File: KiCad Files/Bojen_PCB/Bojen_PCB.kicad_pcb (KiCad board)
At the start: 2 copper layers, 201.9 x 114.3 mm, 9 parts, among them J1 5V Power In, J2 Battery Voltage, U1 Display_TFT_1.8Zoll_ST7735, U2 NEO-GPS8M, U3 SIM800L-CORE, U4 TLP5110 Adafruit Modul, U5 ADS1115 Module, U6 PCF8575 Module, U7 ESP32-DEVKIT-V1

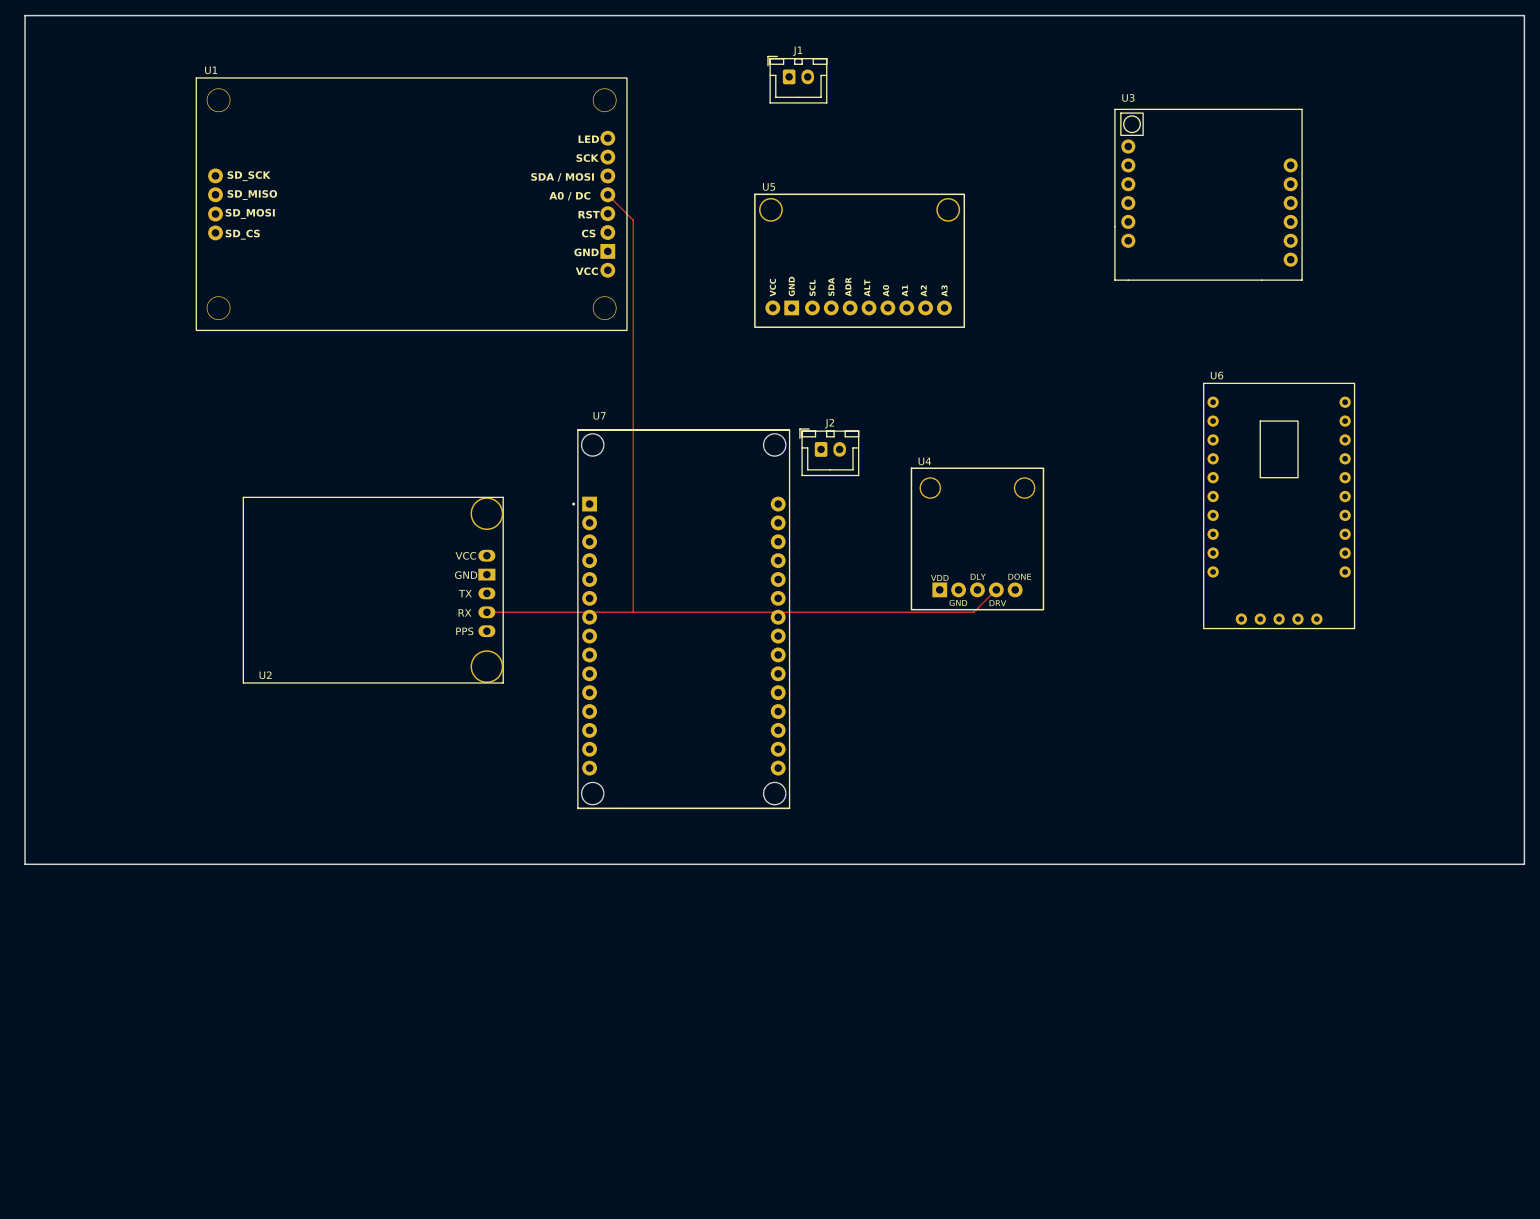
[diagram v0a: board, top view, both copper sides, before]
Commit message: layout
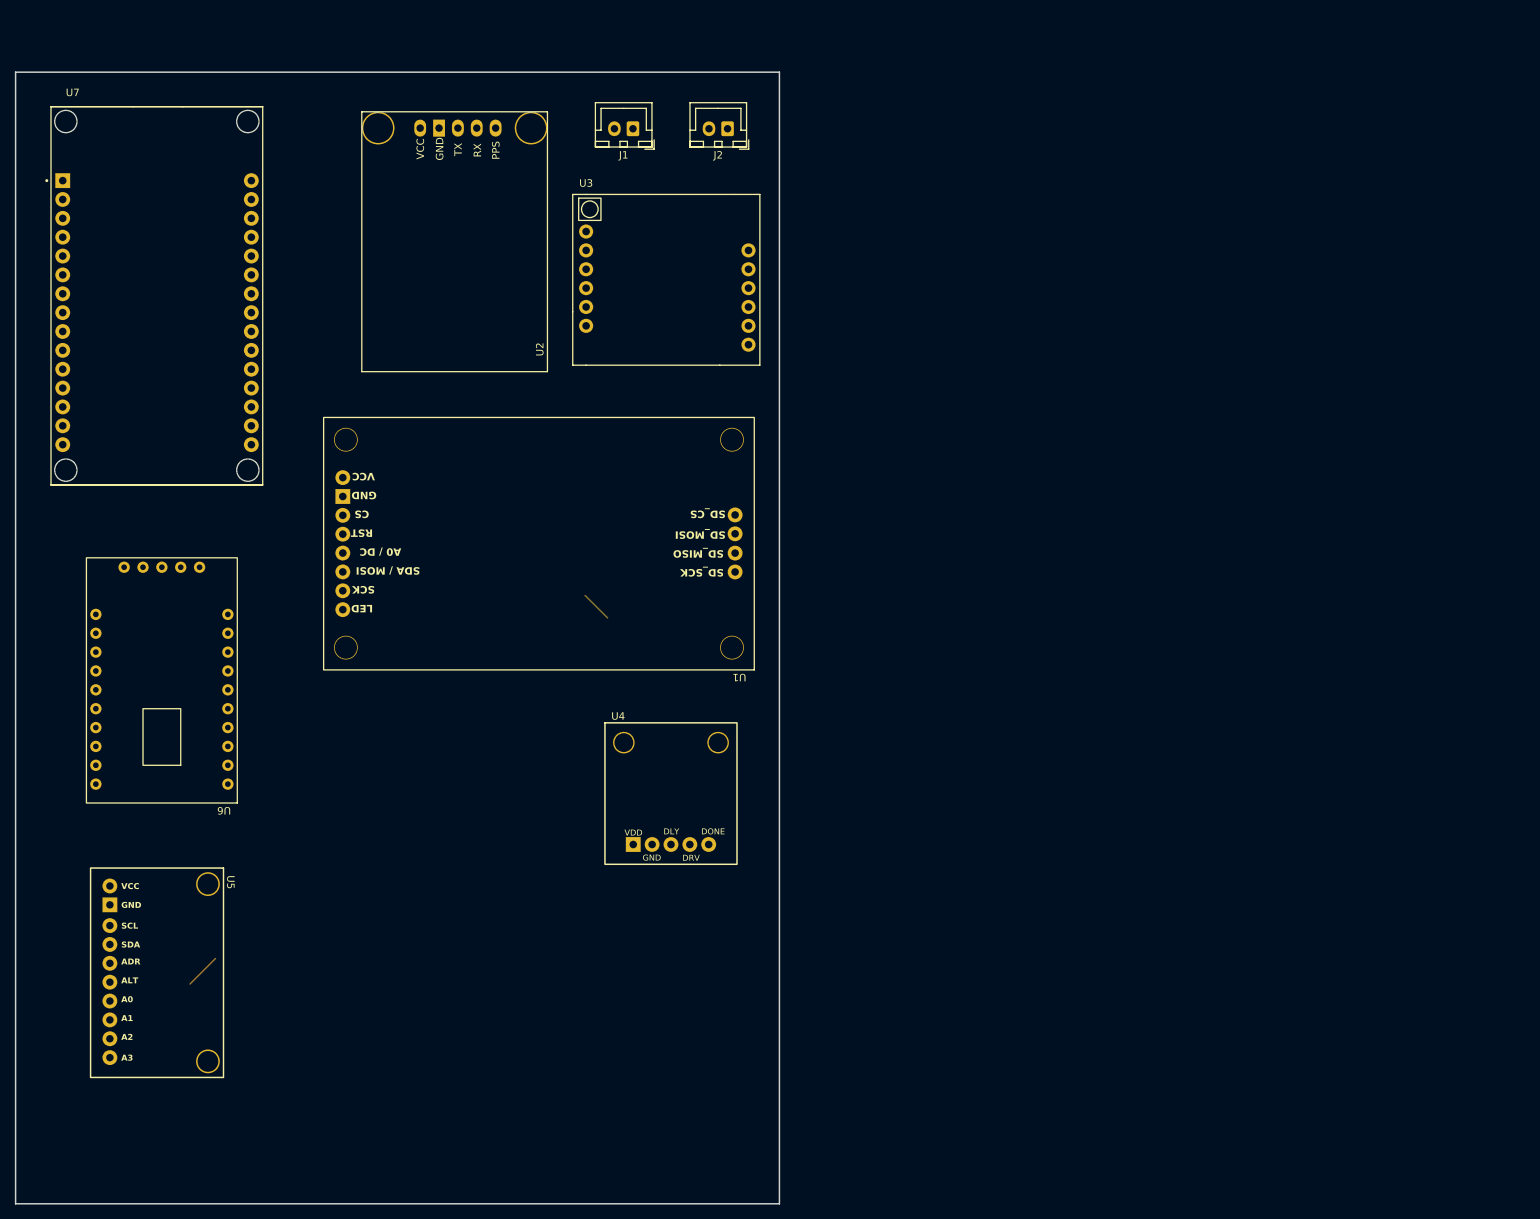
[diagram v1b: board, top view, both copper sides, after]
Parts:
- moved U6 139.6 mm to (69.2, 122.6), turned to 180 degrees
- moved U5 134.7 mm to (57.1, 145.4), turned to -90 degrees
- moved U7 83.3 mm to (57.1, 54.2)
- moved U2 77.2 mm to (109.7, 29.5), turned to 90 degrees
- moved U3 73.9 mm to (114.9, 45.6)
- moved U4 53.7 mm to (126.4, 121.3)
- moved U1 48.8 mm to (108.6, 87.6), turned to 180 degrees
- moved J2 45.0 mm to (134.0, 31.8), turned to 180 degrees
- moved J1 22.2 mm to (121.2, 31.8), turned to 180 degrees
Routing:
- net (no net): track 127.5 -> 0.00 mm
- net unconnected-(U1-TFT_A0_DC-Pad4): track 0.00 -> 4.85 mm
- net Net-(U4-DRV): track 0.00 -> 4.27 mm
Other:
- board size 201.9 x 114.3 mm -> 102.9 x 152.4 mm

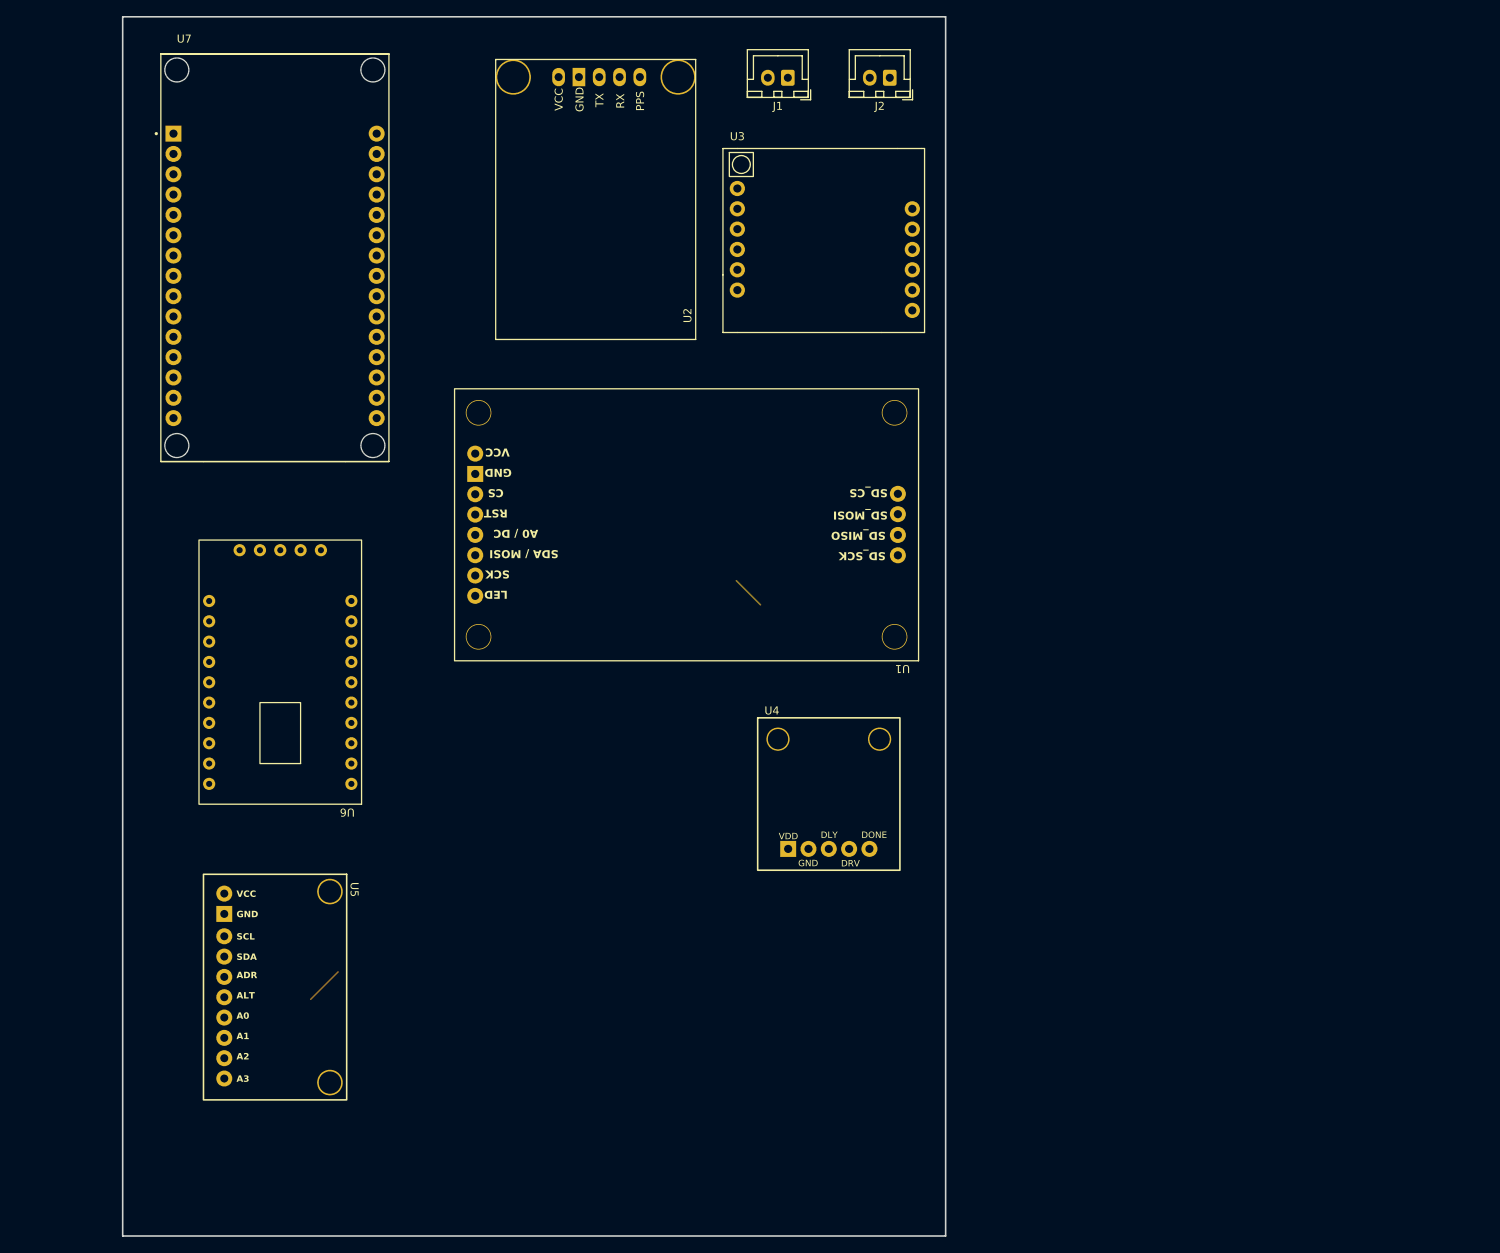
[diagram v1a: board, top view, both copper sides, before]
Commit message: PCB Design
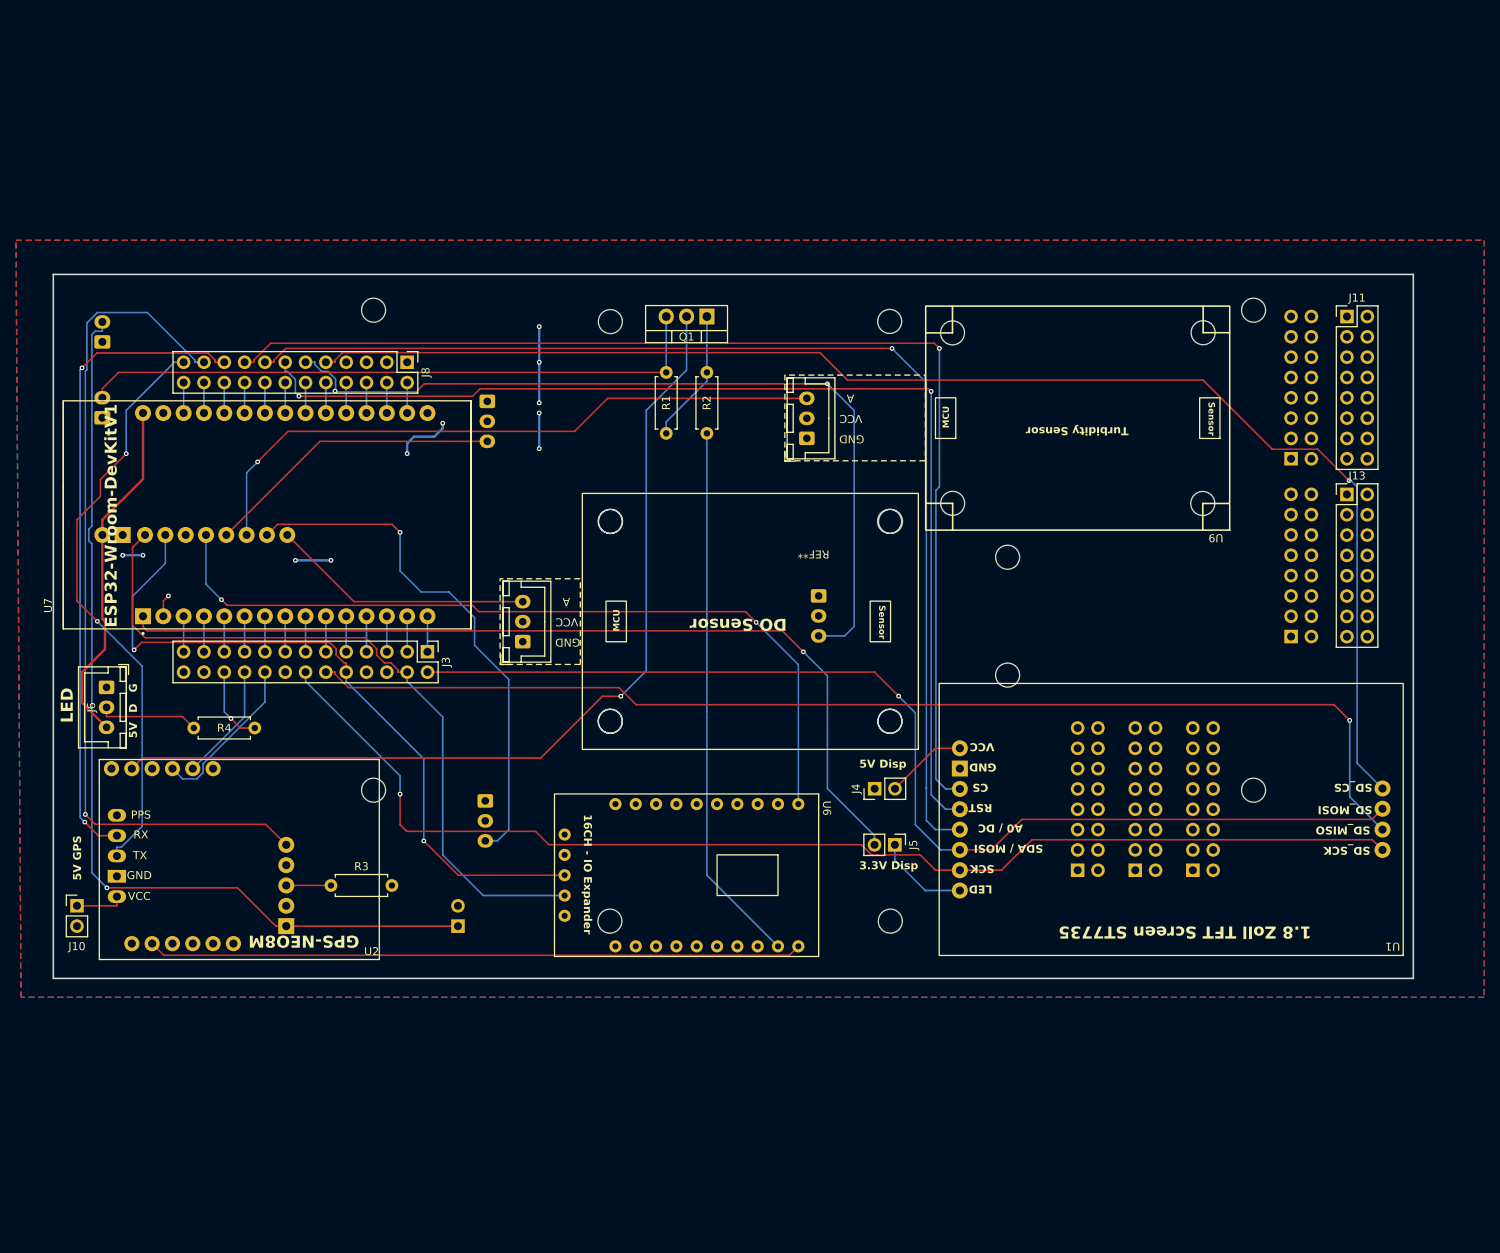
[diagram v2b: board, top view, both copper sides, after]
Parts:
- added J10: GPS EN, Connector_PinHeader_2.54mm:PinHeader_1x02_P2.54mm_Vertical, F.Cu at (32.4, 135.3)
- added J11: Conn_02x08_Odd_Even, Connector_PinHeader_2.54mm:PinHeader_2x08_P2.54mm_Vertical, F.Cu at (191.1, 61.6)
- added J13: Conn_02x08_Odd_Even, Connector_PinHeader_2.54mm:PinHeader_2x08_P2.54mm_Vertical, F.Cu at (191.1, 83.8)
- added J14: Conn_02x08_Odd_Even, Connector_PinHeader_2.54mm:PinHeader_2x08_P2.54mm_Vertical, B.Cu at (184.2, 101.6)
- added J15: Conn_02x08_Odd_Even, Connector_PinHeader_2.54mm:PinHeader_2x08_P2.54mm_Vertical, B.Cu at (184.2, 79.4)
- added J16: Conn_02x08_Odd_Even, Connector_PinHeader_2.54mm:PinHeader_2x08_P2.54mm_Vertical, B.Cu at (157.5, 130.8)
- added J17: Conn_02x08_Odd_Even, Connector_PinHeader_2.54mm:PinHeader_2x08_P2.54mm_Vertical, B.Cu at (164.7, 130.8)
- added J18: Conn_02x08_Odd_Even, Connector_PinHeader_2.54mm:PinHeader_2x08_P2.54mm_Vertical, B.Cu at (171.9, 130.8)
- added J3: GPIO Breakout 2, Connector_PinHeader_2.54mm:PinHeader_2x13_P2.54mm_Vertical, F.Cu at (76.2, 103.5)
- added J4: 5V TFT, Connector_PinHeader_2.54mm:PinHeader_1x02_P2.54mm_Vertical, F.Cu at (132.1, 120.6)
- added J5: 3.3V TFT, Connector_PinHeader_2.54mm:PinHeader_1x02_P2.54mm_Vertical, F.Cu at (134.6, 127.6)
- added J6: LED, Connector_JST:JST_XH_B3B-XH-A_1x03_P2.50mm_Vertical, F.Cu at (36.1, 108.0)
- added J8: GPIO Breakout 1, Connector_PinHeader_2.54mm:PinHeader_2x12_P2.54mm_Vertical, F.Cu at (73.7, 67.3)
- added J9: PWR TMR SKIP, Connector_PinHeader_2.54mm:PinHeader_1x02_P2.54mm_Vertical, B.Cu at (80.0, 137.8)
- added Q1: IRF5210PBF, Package_TO_SOT_THT:TO-220-3_Vertical, F.Cu at (111.1, 61.6)
- added R1: 10k, Resistor_THT:R_Axial_DIN0207_L6.3mm_D2.5mm_P7.62mm_Horizontal, F.Cu at (106.0, 68.6)
- added R2: 470, Resistor_THT:R_Axial_DIN0207_L6.3mm_D2.5mm_P7.62mm_Horizontal, F.Cu at (111.1, 76.2)
- added R3: 220k, Resistor_THT:R_Axial_DIN0207_L6.3mm_D2.5mm_P7.62mm_Horizontal, F.Cu at (64.1, 132.7)
- added R4: 330, Resistor_THT:R_Axial_DIN0207_L6.3mm_D2.5mm_P7.62mm_Horizontal, F.Cu at (47.0, 113.0)
- added REF**: Battery Footprint, Datenbojen:Battery Footprint, F.Cu at (124.5, 90.8)
- added U10: PH Sensor, Datenbojen:PH Sensor DFRobot, B.Cu at (116.5, 124.7)
- added U11: DO Sensor, Datenbojen:DO Sensor DFRobot, F.Cu at (116.6, 99.7)
- added U12: TMP Sensor, Datenbojen:Tempterature Sensor DFRobot, B.Cu at (153.5, 99.0)
- added U8: TDS Sensor, Datenbojen:TDS Sensor DFRobot, B.Cu at (116.5, 74.7)
- added U9: Turbidity Sensor, Datenbojen:Turbidity Sensor DFRobot, F.Cu at (157.5, 74.3)
- J1, J2, U3: moved to B.Cu
- U1: footprint Datenbojen:ST7735 TFT Screen 1.8 Zoll -> Datenbojen:ST7735 TFT Screen 1.8 Zoll no hole
- U2: footprint Datenbojen:GY-NEO8MV2 -> Datenbojen:GY-NEO8MV2 no hole
- U4: value TLP5110 Adafruit Modul -> TLP5110 Power Timer Modul; footprint Datenbojen:TPL5110 Board -> Datenbojen:TPL5110 Board no hole; moved to B.Cu
- U5: value ADS1115 Module -> ADC - ADS1115 Module; footprint Datenbojen:ADS1115 Module -> Datenbojen:ADC - ADS1115 Module no hole; moved to B.Cu
- U7: footprint Datenbojen:MODULE_ESP32_DEVKIT_V1 -> Datenbojen:MODULE_ESP32_DEVKIT_V1 no hole
- moved U2 115.0 mm to (35.2, 117.0), turned to 180 degrees
- moved J2 107.2 mm to (35.6, 74.3), turned to 90 degrees
- moved U3 106.7 mm to (36.7, 118.1), turned to -90 degrees
- moved J1 91.8 mm to (35.6, 64.8), turned to 90 degrees
- moved U1 70.9 mm to (169.2, 124.5)
- moved U4 62.0 mm to (65.4, 132.7), turned to 90 degrees
- moved U6 55.9 mm to (125.1, 120.0), turned to -90 degrees
- moved U5 51.1 mm to (47.2, 95.2), turned to 0 degrees
- moved U7 32.1 mm to (56.2, 86.4), turned to 90 degrees
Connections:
- J2 pad 1: unconnected-(J2-Pin_1-Pad1) -> GND
- J2 pad 2: unconnected-(J2-Pin_2-Pad2) -> +BATT
- U1 pad 1: unconnected-(U1-TFT_LED-Pad1) -> Net-(J5-Pin_1)
- U1 pad 10: unconnected-(U1-SD_MOSI-Pad10) -> /SPI_MOSI
- U1 pad 11: unconnected-(U1-SD_MISO-Pad11) -> /SPI_MISO
- U1 pad 12: unconnected-(U1-SD_SCK-Pad12) -> /SPI_SCK
- U1 pad 2: unconnected-(U1-TFT_SCK-Pad2) -> /SPI_SCK
- U1 pad 3: unconnected-(U1-TFT_SDA_MOSI-Pad3) -> /SPI_MOSI
- U1 pad 4: unconnected-(U1-TFT_A0_DC-Pad4) -> /TFT_DC
- U1 pad 5: unconnected-(U1-TFT_RST-Pad5) -> /TFT_RST
- U1 pad 6: unconnected-(U1-TFT_CS-Pad6) -> /TFT_CS
- U1 pad 7: unconnected-(U1-GND-Pad7) -> GND
- U1 pad 8: unconnected-(U1-VCC-Pad8) -> Net-(J4-Pin_2)
- U1 pad 9: unconnected-(U1-SD_CS-Pad9) -> /SD_CS
- U2 pad 1: unconnected-(U2-VCC-Pad1) -> Net-(J10-Pin_1)
- U2 pad 2: unconnected-(U2-GND-Pad2) -> GND
- U2 pad 3: unconnected-(U2-TX-Pad3) -> /RX1
- U2 pad 4: unconnected-(U2-RX-Pad4) -> /TX1
- U3 pad 11: unconnected-(U3-DTR-Pad11) -> /SIM_DTR
- U3 pad 2: unconnected-(U3-VCC-Pad2) -> Net-(Q1-D)
- U3 pad 4: unconnected-(U3-RXD-Pad4) -> /TX2
- U3 pad 5: unconnected-(U3-TXD-Pad5) -> /RX2
- U3 pad 6: unconnected-(U3-GND-Pad6) -> GND
- U4 pad 3: unconnected-(U4-Delay-Pad3) -> Net-(U4-Delay)
- U4 pad 4: Net-(U4-DRV) -> +5V
- U4 pad 5: unconnected-(U4-Done-Pad5) -> /PWR_Done
- U5 pad 1: unconnected-(U5-VCC-Pad1) -> +5V
- U5 pad 10: unconnected-(U5-A3-Pad10) -> /ADC3
- U5 pad 2: unconnected-(U5-GND-Pad2) -> GND
- U5 pad 3: unconnected-(U5-SCL-Pad3) -> /I2C_SCL
- U5 pad 4: unconnected-(U5-SDA-Pad4) -> /I2C_SDA
- U5 pad 6: unconnected-(U5-ALRT-Pad6) -> /ADC_ALRT
- U5 pad 7: unconnected-(U5-A0-Pad7) -> /ADC0
- U5 pad 8: unconnected-(U5-A1-Pad8) -> /ADC1
- U5 pad 9: unconnected-(U5-A2-Pad9) -> /ADC2
- U6 pad 1: unconnected-(U6-P10-Pad1) -> /ADC_ALRT
- U6 pad 19: unconnected-(U6-P06-Pad19) -> /~SIM_EN
- U6 pad 20: unconnected-(U6-P07-Pad20) -> /SIM_DTR
- U6 pad C1: unconnected-(U6-GND-PadC1) -> GND
- U6 pad C2: unconnected-(U6-VCC-PadC2) -> +5V
- U6 pad C3: unconnected-(U6-SDA-PadC3) -> /I2C_SDA
- U6 pad C4: unconnected-(U6-SCL-PadC4) -> /I2C_SCL
- U7 pad 1: unconnected-(U7-3V3-Pad1) -> +3.3V
- U7 pad 10: unconnected-(U7-D19-Pad10) -> /ESP32/D19
- U7 pad 11: unconnected-(U7-D21-Pad11) -> /ESP32/D21
- U7 pad 12: unconnected-(U7-RX0-Pad12) -> /ESP32/RX0
- U7 pad 13: unconnected-(U7-TX0-Pad13) -> /ESP32/TX0
- U7 pad 14: unconnected-(U7-D22-Pad14) -> /ESP32/D22
- U7 pad 15: unconnected-(U7-D23-Pad15) -> /ESP32/D23
- U7 pad 17: unconnected-(U7-VP-Pad17) -> /ESP32/VP
- U7 pad 18: unconnected-(U7-VN-Pad18) -> /ESP32/VN
- U7 pad 19: unconnected-(U7-D34-Pad19) -> /ESP32/D34
- U7 pad 2: Net-(U7-GND-Pad2) -> GND
- U7 pad 20: unconnected-(U7-D35-Pad20) -> /ESP32/D35
- U7 pad 21: unconnected-(U7-D32-Pad21) -> /ESP32/D32
- U7 pad 22: unconnected-(U7-D33-Pad22) -> /ESP32/D33
- U7 pad 23: unconnected-(U7-D25-Pad23) -> /ESP32/D25
- U7 pad 24: unconnected-(U7-D26-Pad24) -> /ESP32/D26
- U7 pad 25: unconnected-(U7-D27-Pad25) -> /ESP32/D27
- U7 pad 26: unconnected-(U7-D14-Pad26) -> /ESP32/D14
- U7 pad 27: unconnected-(U7-D12-Pad27) -> /ESP32/D12
- U7 pad 28: unconnected-(U7-D13-Pad28) -> /ESP32/D13
- U7 pad 29: Net-(U7-GND-Pad2) -> GND
- U7 pad 3: unconnected-(U7-D15-Pad3) -> /ESP32/D15
- U7 pad 30: Net-(U4-DRV) -> +5V
- U7 pad 4: unconnected-(U7-D2-Pad4) -> /ESP32/D2
- U7 pad 5: unconnected-(U7-D4-Pad5) -> /ESP32/D4
- U7 pad 6: unconnected-(U7-RX2-Pad6) -> /ESP32/RX2
- U7 pad 7: unconnected-(U7-TX2-Pad7) -> /ESP32/TX2
- U7 pad 8: unconnected-(U7-D5-Pad8) -> /ESP32/D5
- U7 pad 9: unconnected-(U7-D18-Pad9) -> /ESP32/D18
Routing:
- net /SD_CS: track 0.00 -> 175.5 mm, vias 0 -> 1
- net /SPI_SCK: track 0.00 -> 151.2 mm, vias 0 -> 1
- net /SPI_MISO: track 0.00 -> 146.0 mm, vias 0 -> 1
- net /TFT_CS: track 0.00 -> 145.8 mm, vias 0 -> 1
- net /TFT_DC: track 0.00 -> 144.7 mm, vias 0 -> 1
- net /TFT_RST: track 0.00 -> 139.4 mm, vias 0 -> 2
- net /SPI_MOSI: track 0.00 -> 138.9 mm, vias 0 -> 1
- net Net-(J1-Pin_2): track 0.00 -> 118.8 mm, vias 0 -> 1
- net Net-(Q1-D): track 0.00 -> 115.7 mm, vias 0 -> 1
- net +3.3V: track 0.00 -> 113.0 mm, vias 0 -> 1
- net /PWR_Done: track 0.00 -> 106.1 mm, vias 0 -> 1
- net /TMP_SENS: track 0.00 -> 105.0 mm, vias 0 -> 2
- net /ADC_ALRT: track 0.00 -> 101.8 mm, vias 0 -> 2
- net /I2C_SCL: track 0.00 -> 91.4 mm
- net /I2C_SDA: track 0.00 -> 90.2 mm, vias 0 -> 2
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- added copper zone on B.Cu, net +5V
- added copper zone on F.Cu, net GND
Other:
- board size 102.9 x 152.4 mm -> 170 x 88 mm
- board text added: "3.3V Disp"
- board text added: "5V"
- board text added: "5V Disp"
- board text added: "5V GPS"
- board text added: "Beidseitiges Löten mit Pin Sockets"
- board text added: "D"
- board text added: "G"
- board text added: "LED"
- board text added: "PWR Timer Skip"
- board text added: "UP"
